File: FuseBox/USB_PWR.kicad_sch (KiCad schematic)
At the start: 54 parts, among them J1 UJ31CHG2SMTTR, U1 TPS61040DBVR, U2 LT3030EFETRPBF

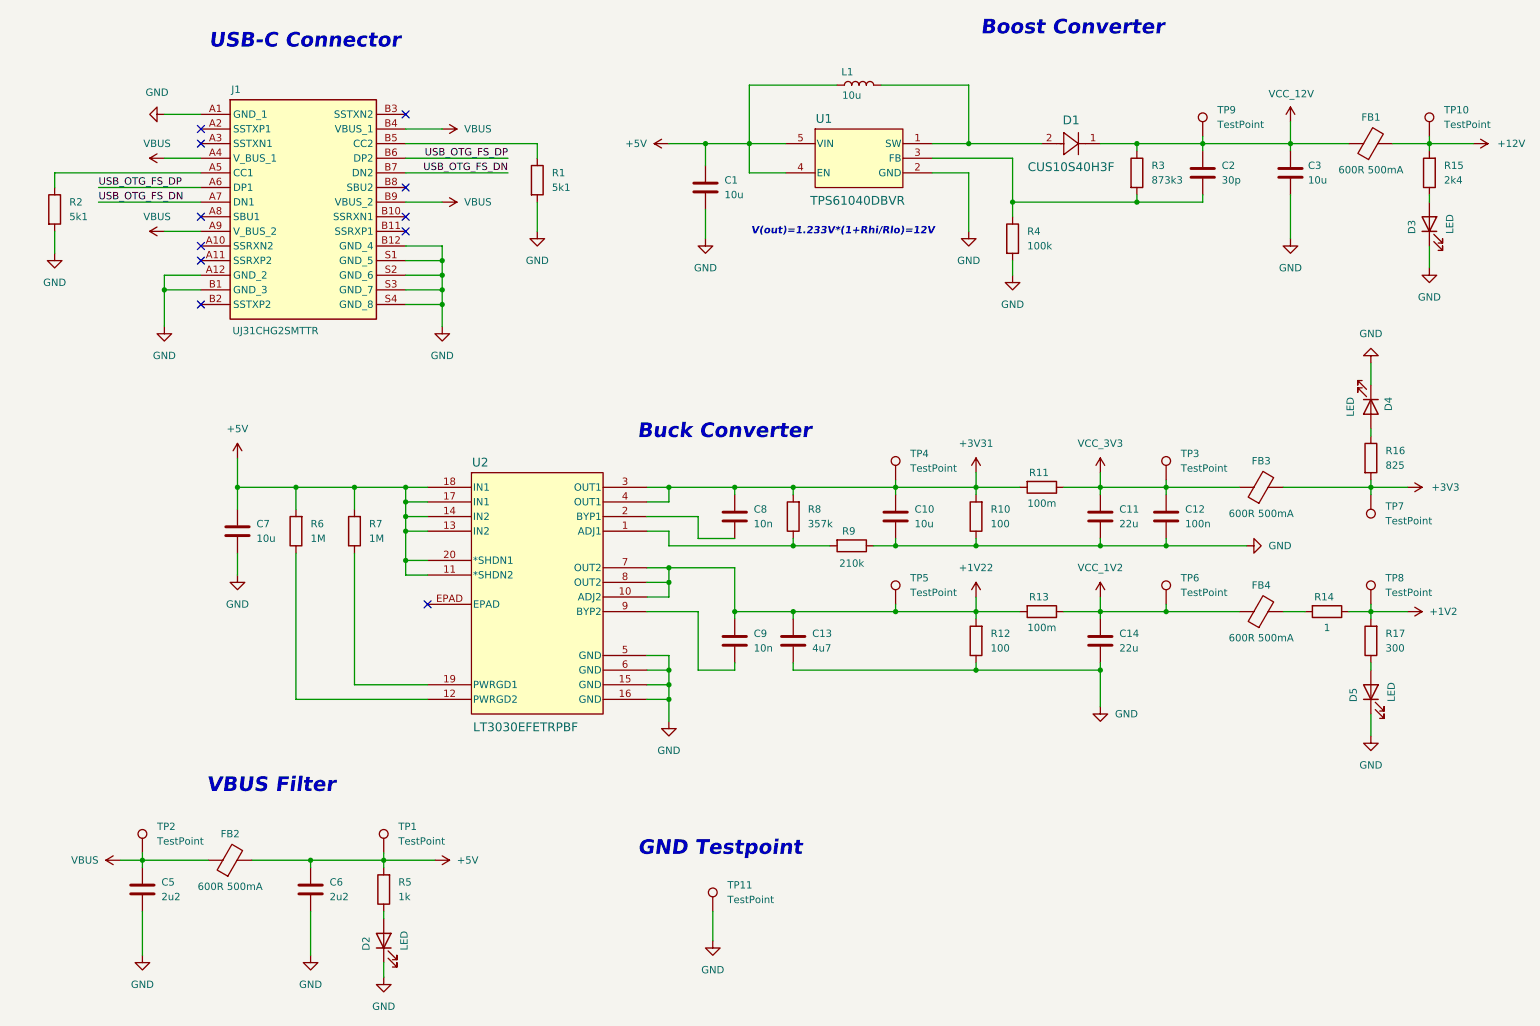
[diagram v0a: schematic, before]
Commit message: changes
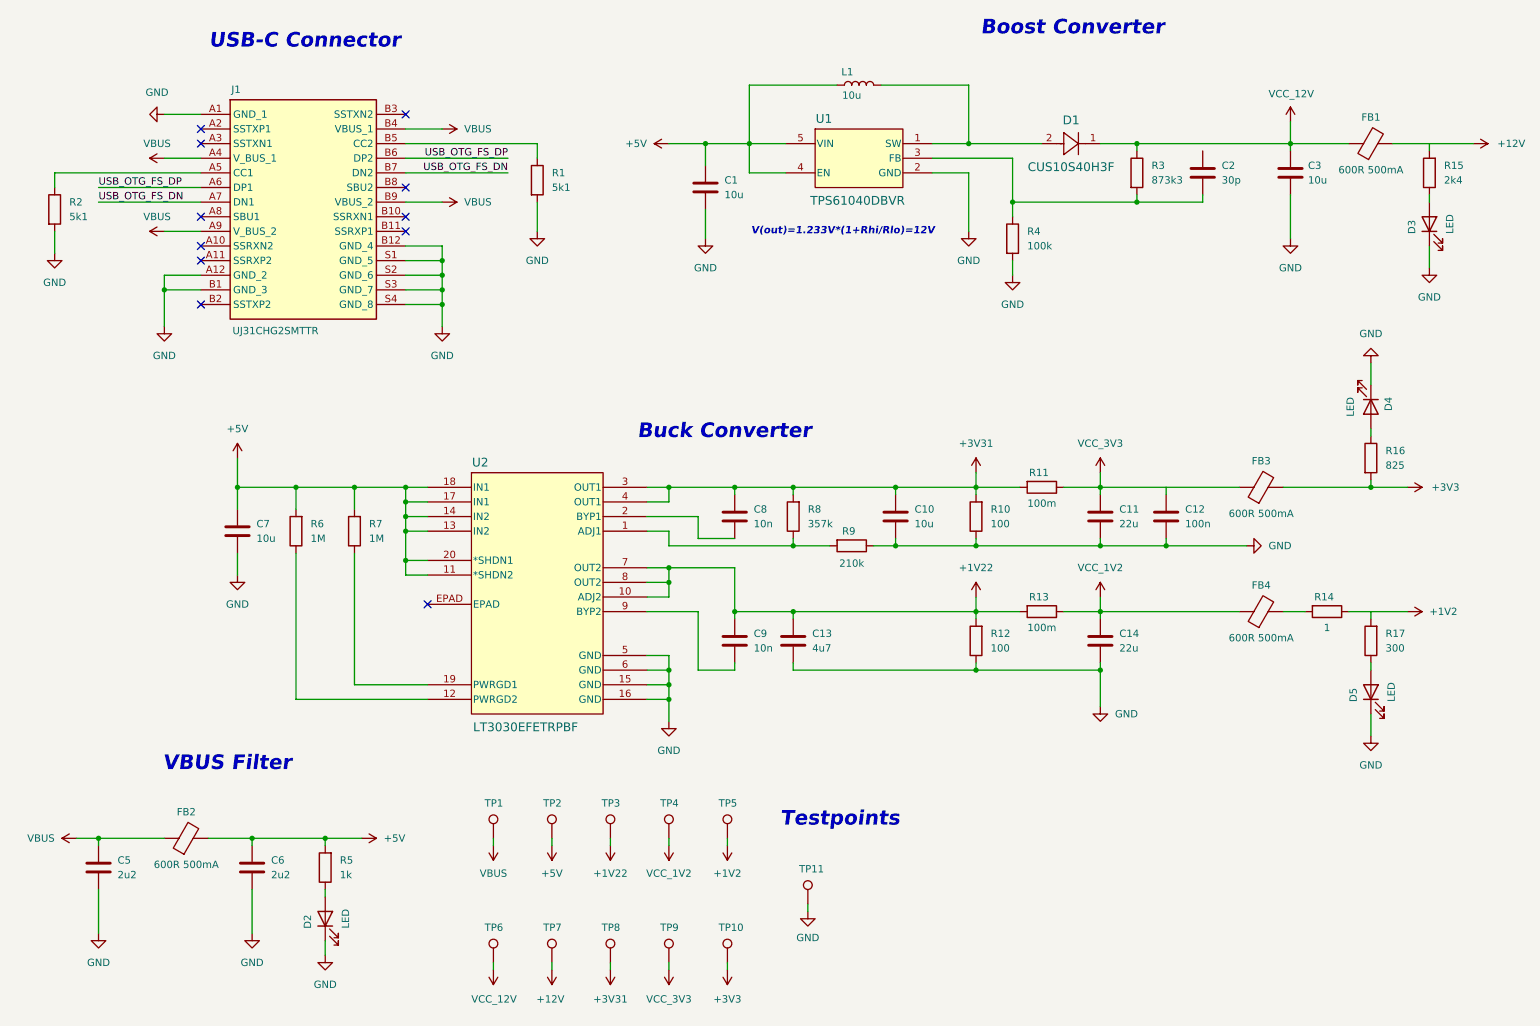
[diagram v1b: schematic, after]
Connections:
- net +12V: now also TP7.1; no longer R15.2, TP10.1
- net +1V2: now also TP5.1; no longer R17.2, TP8.1
- net +1V22: now also TP3.1; no longer TP5.1
- net +3V3: now also TP10.1; no longer TP7.1
- net +3V31: now also TP8.1; no longer TP4.1
- net +5V: now also TP2.1; no longer TP1.1
- net VBUS: now also TP1.1; no longer TP2.1
- net VCC_12V: now also TP6.1; no longer C2.1, TP9.1
- net VCC_1V2: now also TP4.1; no longer TP6.1
- net VCC_3V3: now also TP9.1; no longer C12.1, TP3.1
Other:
- note added: "Testpoints"
- note removed: "GND Testpoint"
- moved on the sheet: C5, C6, D2, FB2, R5, TP1

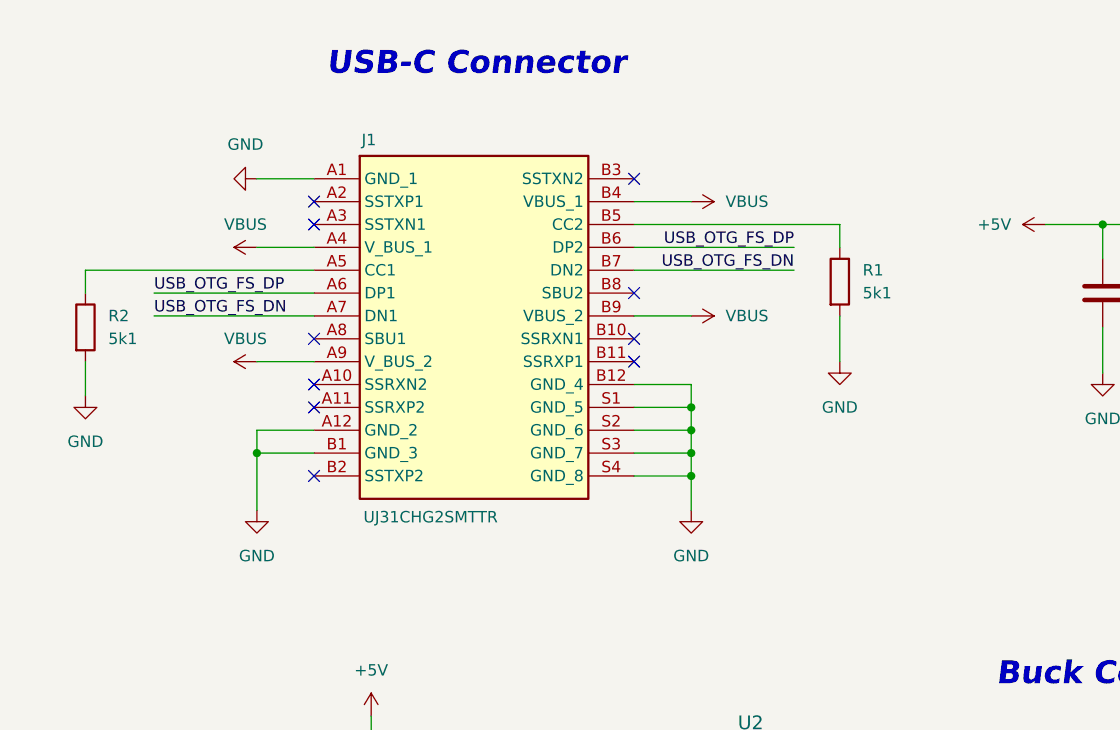
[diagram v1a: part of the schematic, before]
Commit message: changes
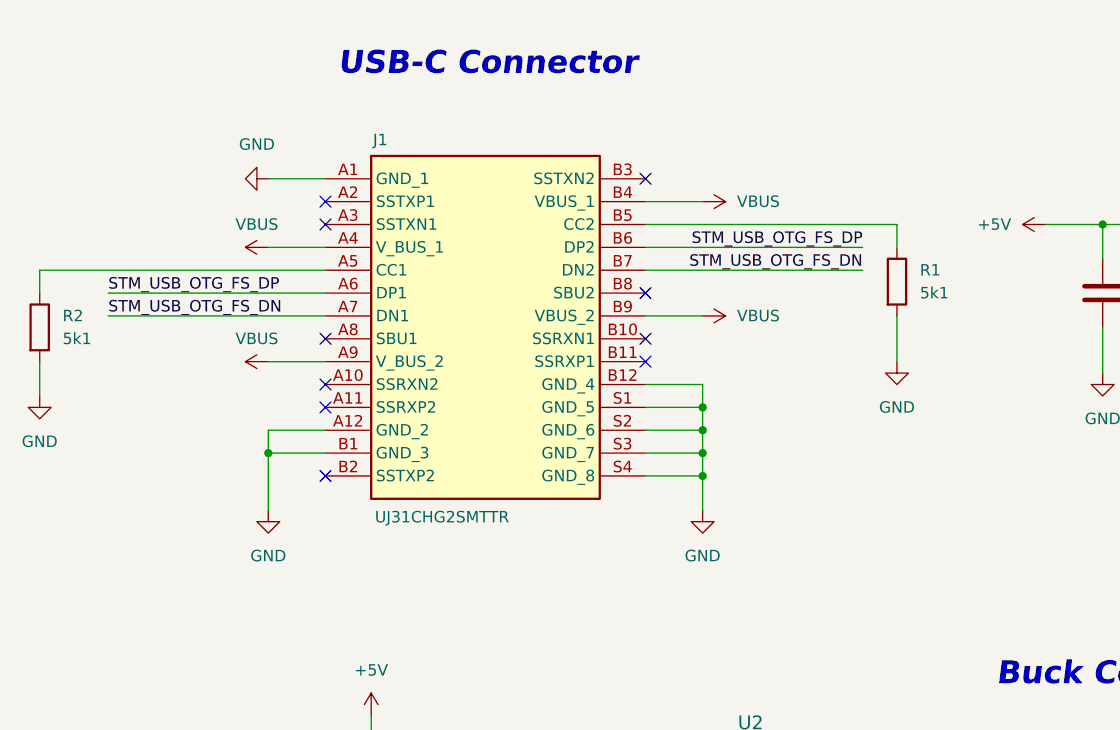
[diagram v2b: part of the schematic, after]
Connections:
- net USB_OTG_FS_DN renamed STM_USB_OTG_FS_DN
- net USB_OTG_FS_DP renamed STM_USB_OTG_FS_DP
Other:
- moved on the sheet: J1, R1, R2
